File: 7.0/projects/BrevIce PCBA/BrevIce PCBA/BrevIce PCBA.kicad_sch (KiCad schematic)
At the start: 12 parts, among them J1 Conn_01x04_Socket, J2 Conn_01x05_Socket, J3 Conn_01x03_Socket, K1 Relay_SPDT, K2 Relay_SPDT, Q1 AO3400A, Q2 AO3400A, U1 ATmega3208-X

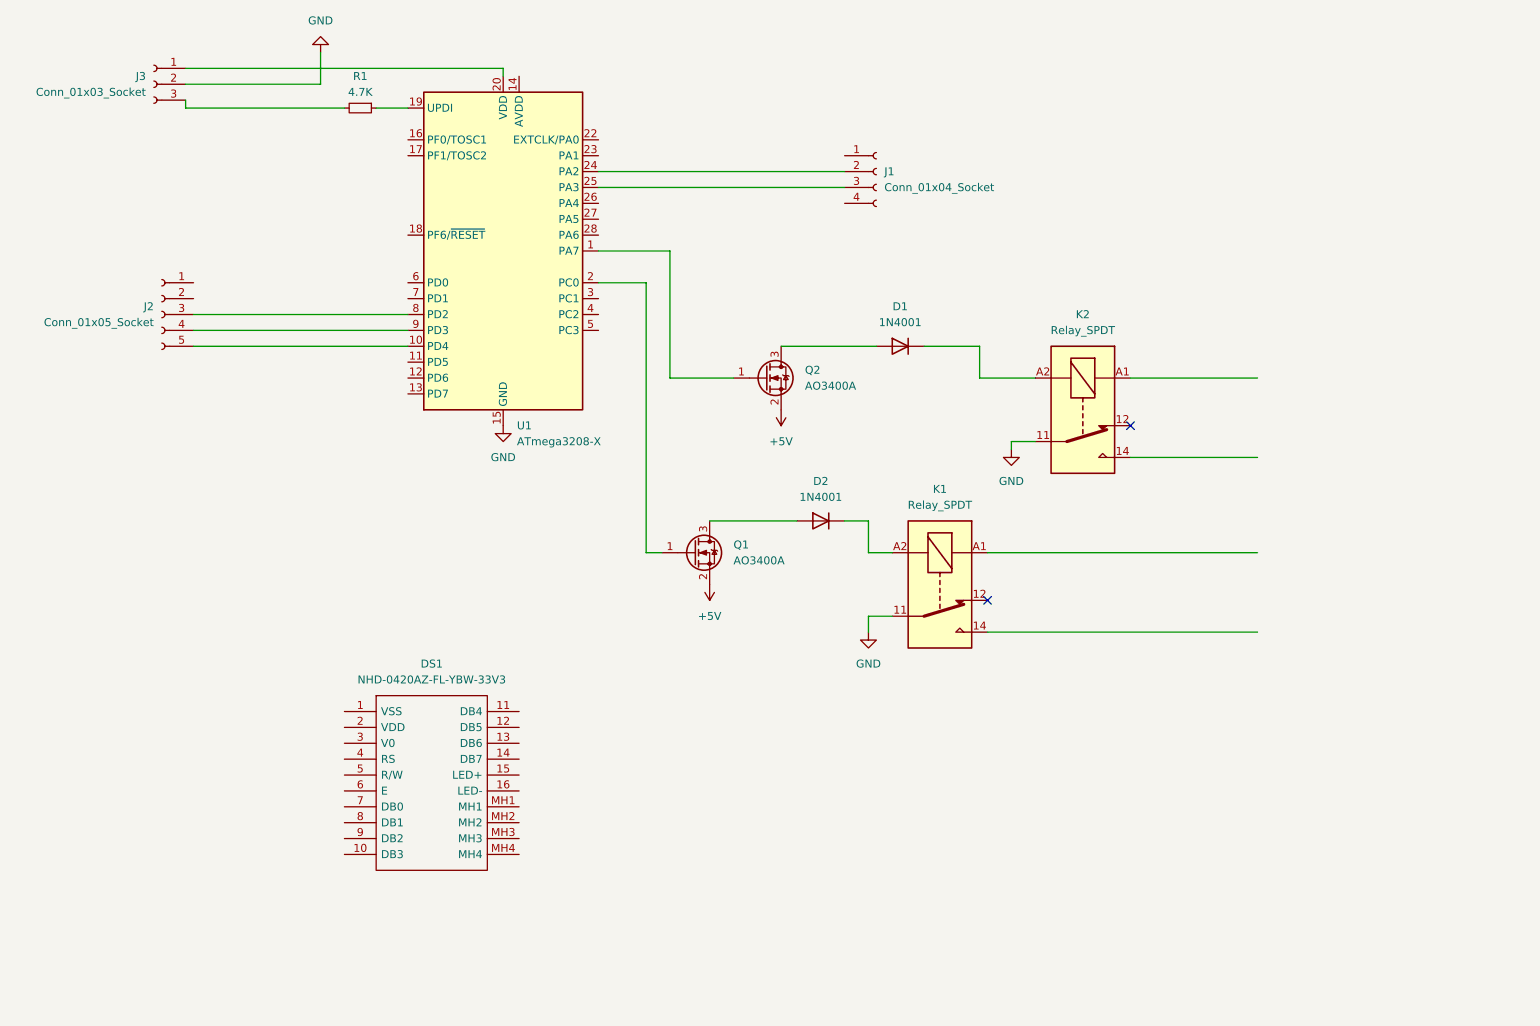
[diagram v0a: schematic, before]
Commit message: Update
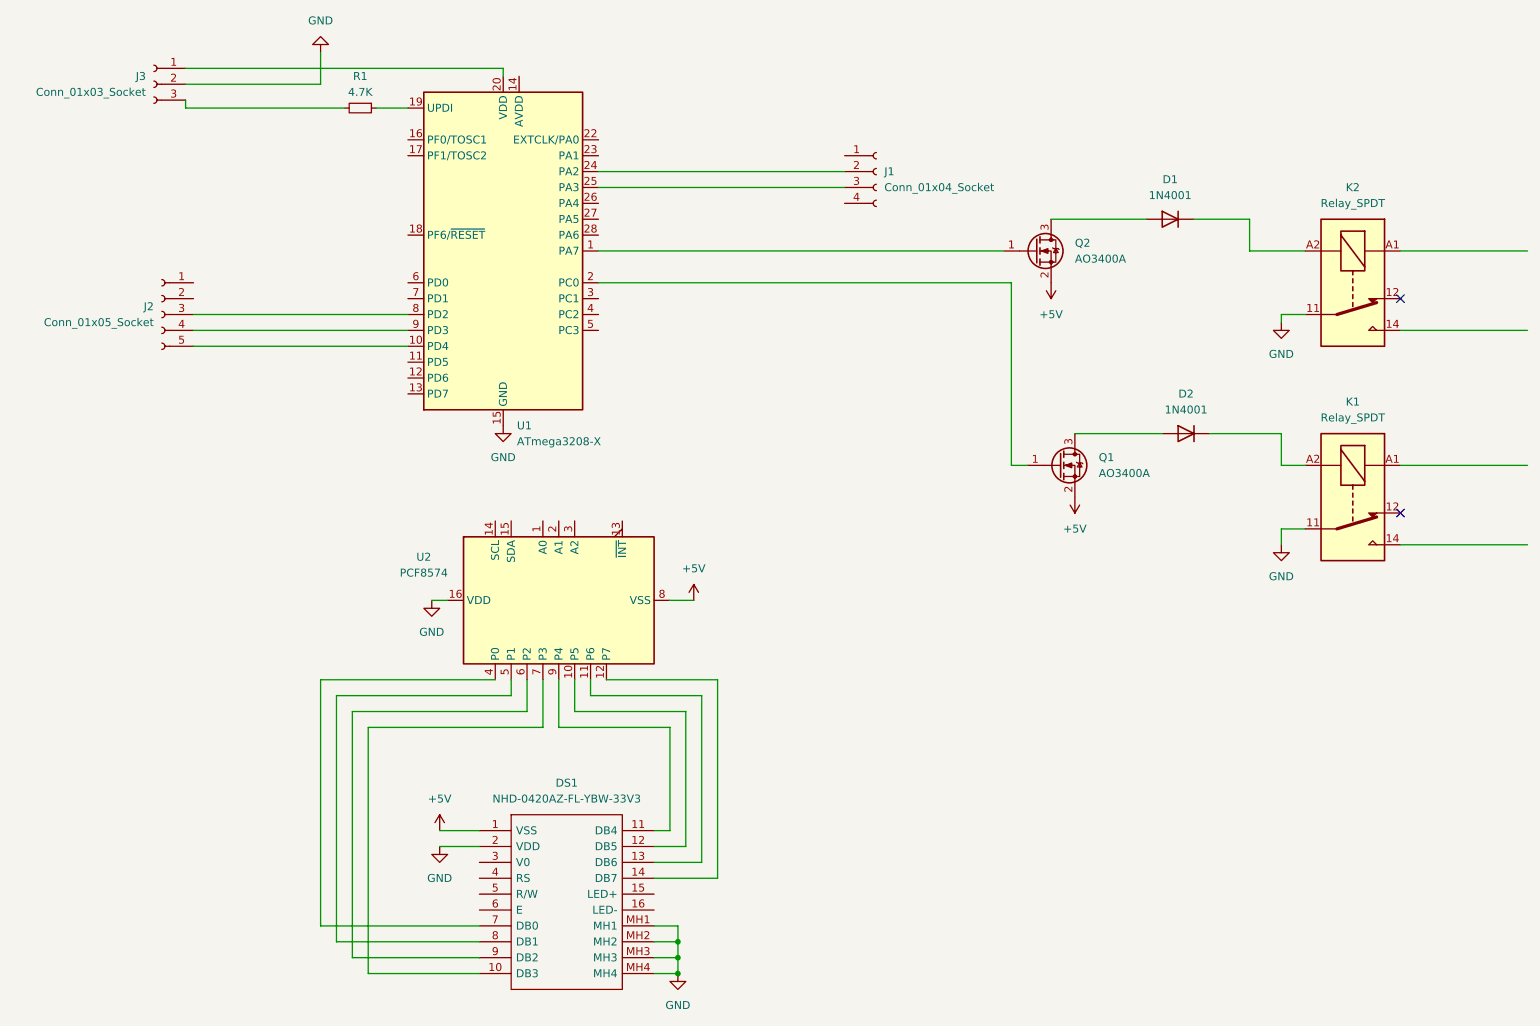
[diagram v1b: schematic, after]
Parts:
- added U2: PCF8574, symbol Interface_Expansion:PCF8574
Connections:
- net +5V: now also DS1.1 (VSS), U2.8 (VSS)
- net GND: now also DS1.2 (VDD), DS1.MH1, DS1.MH2, DS1.MH3, DS1.MH4, U2.16 (VDD)
- net at DS1.10 (DB3): now also U2.7 (P3)
- net at DS1.11 (DB4): now also U2.9 (P4)
- net at DS1.12 (DB5): now also U2.10 (P5)
- net at DS1.13 (DB6): now also U2.11 (P6)
- net at DS1.14 (DB7): now also U2.12 (P7)
- net at DS1.7 (DB0): now also U2.4 (P0)
- net at DS1.8 (DB1): now also U2.5 (P1)
- net at DS1.9 (DB2): now also U2.6 (P2)
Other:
- moved on the sheet: D1, D2, DS1, K1, K2, Q1, Q2
